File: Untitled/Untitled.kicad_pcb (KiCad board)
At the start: 2 copper layers, 12 x 16.4 mm, 13 parts, among them J1 USB_A, U1 AP7333-33SRG-7, U2 ESP32-C3, Y1 Crystal_GND24_Small

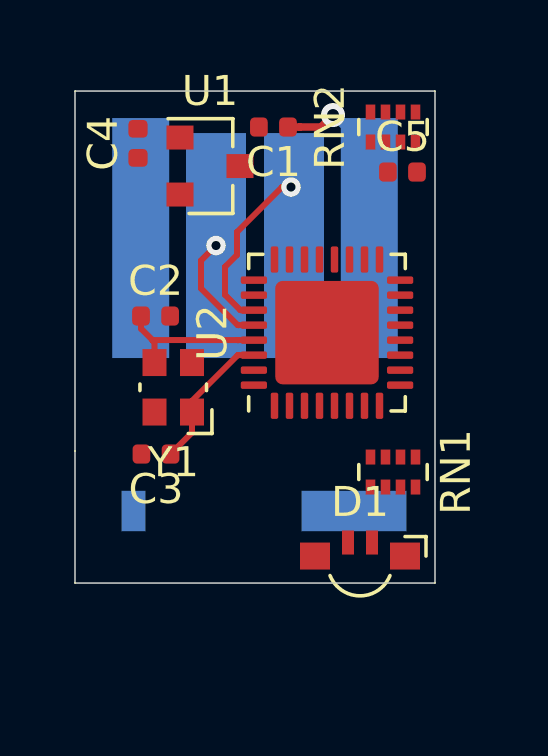
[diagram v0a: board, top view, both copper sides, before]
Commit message: morr work
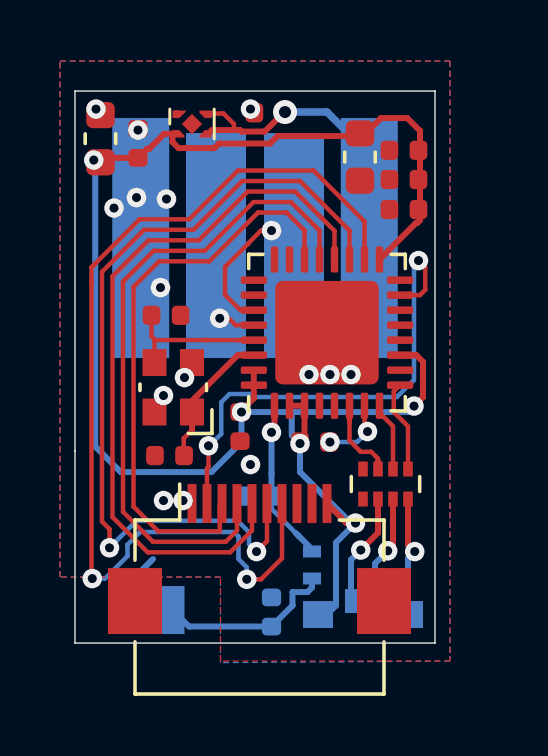
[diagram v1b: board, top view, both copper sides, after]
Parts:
- removed RN2: R_Pack04, Resistor_SMD:R_Array_Concave_4x0402
- added C10: C_Small, Capacitor_SMD:C_0603_1608Metric, F.Cu at (142.3, 38.6)
- added C11: C_Small, Capacitor_SMD:C_0402_1005Metric, B.Cu at (148.1, 54.4)
- added C12: C_Small, Capacitor_SMD:C_0402_1005Metric, B.Cu at (147.7, 50.5)
- added C6: C_Small, Capacitor_SMD:C_0402_1005Metric, F.Cu at (152.5, 40.0)
- added C7: C_Small, Capacitor_SMD:C_0402_1005Metric, F.Cu at (152.5, 41.0)
- added C8: C_Small, Capacitor_SMD:C_0402_1005Metric, F.Cu at (152.5, 39.0)
- added C9: C_Small, Capacitor_SMD:C_0603_1608Metric, F.Cu at (151.0, 39.2)
- added J2: Conn_02x05_Odd_Even, Connector_FFC-FPC:Hirose_FH12-10S-0.5SH_1x10-1MP_P0.50mm_Horizontal, F.Cu at (147.7, 52.6)
- added L1: L_Small, Inductors_SMD:L_0402, B.Cu at (149.4, 52.8)
- added R1: R_Small, Resistor_SMD:R_0402_1005Metric, F.Cu at (149.5, 48.7)
- AE1: footprint footprint:ACAG0801-2450Trecudedkeepout -> footprint:Antenna-AVX-1001312
- D1: moved to B.Cu
- U1: footprint Package_TO_SOT_SMD:SOT-23 -> Housings_DFN_QFN:UDFN-4_1x1mm_Pitch0.65mm
- moved C5 10.1 mm to (147.0, 48.2), turned to 270 degrees
- moved AE1 3.97 mm to (144.0, 54.2), turned to 180 degrees
- moved D1 1.95 mm to (151.1, 54.5), turned to 0 degrees
- moved U1 1.52 mm to (145.4, 38.1)
- moved C1 0.50 mm to (148.0, 37.7)
- moved RN1 0.47 mm to (151.8, 50.1)
- moved C3 0.45 mm to (144.7, 49.1)
- moved C2 0.35 mm to (144.5, 44.5)
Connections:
- net Net-(U2-Pad16) renamed /GP10
- net Net-(U2-Pad25) renamed /URX
- net Net-(U2-Pad26) renamed /UTX
- AE1 pad 2: (no net) -> GND
- C5 pad 1: Net-(C5-Pad1) -> +3V3
- C5 pad 2: Net-(C5-Pad2) -> GND
- J1 pad 4: Net-(J1-Pad4) -> GND
- U2 pad 1: Net-(AE1-Pad1) -> Net-(C12-Pad2)
- U2 pad 18: Net-(U2-Pad18) -> /GP11
- U2 pad 19: Net-(U2-Pad19) -> /GP12
- U2 pad 20: Net-(U2-Pad20) -> /GP13
- U2 pad 21: Net-(U2-Pad21) -> /GP14
- U2 pad 22: Net-(U2-Pad22) -> /GP15
- U2 pad 6: /LED_R -> /LED_B
- U2 pad 9: /LED_B -> /LED_R
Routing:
- net +3V3: track 0.00 -> 55.2 mm, vias 0 -> 5
- net /GP11: track 0.00 -> 33.5 mm, vias 0 -> 2
- net /GP12: track 0.00 -> 28.1 mm, vias 0 -> 2
- net /GP13: track 0.00 -> 24.4 mm
- net /GP14: track 0.00 -> 21.9 mm
- net /GP15: track 0.00 -> 19.4 mm
- net /BLSEL: track 0.00 -> 16.4 mm, vias 0 -> 2
- net Net-(C12-Pad2): track 0.00 -> 6.32 mm, vias 0 -> 1
- net Net-(AE1-Pad1): track 0.00 -> 5.98 mm
- net Net-(D1-Pad2): track 0.00 -> 4.04 mm, vias 0 -> 1
- net VBUS: track 6.27 -> 10.3 mm
- net Net-(D1-Pad4): track 0.00 -> 3.77 mm, vias 0 -> 1
- net Net-(D1-Pad3): track 0.00 -> 3.65 mm, vias 0 -> 1
- net /LED_B: track 0.00 -> 3.27 mm
- net /LED_R: track 0.00 -> 3.08 mm
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- added copper zone on B.Cu, net GND
- added copper zone on F.Cu, net GND
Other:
- board size 12 x 16.4 mm -> 12 x 18.4 mm
